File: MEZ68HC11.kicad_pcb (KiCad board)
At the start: 2 copper layers, 99.1 x 85.2 mm, 29 parts, among them J1 Conn_01x20_Socket, J2 Conn_01x20_Socket, J3 Barrel_Jack_Switch, J4 Conn_01x06_Pin, J5 Conn_01x08_Pin, J7 PinHeader_1x06_P2.54mm_Vertic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, SW1 SW_SPDT, SW2 SW_SPST, U1 PIC18F47Q43-IP, U2 628128

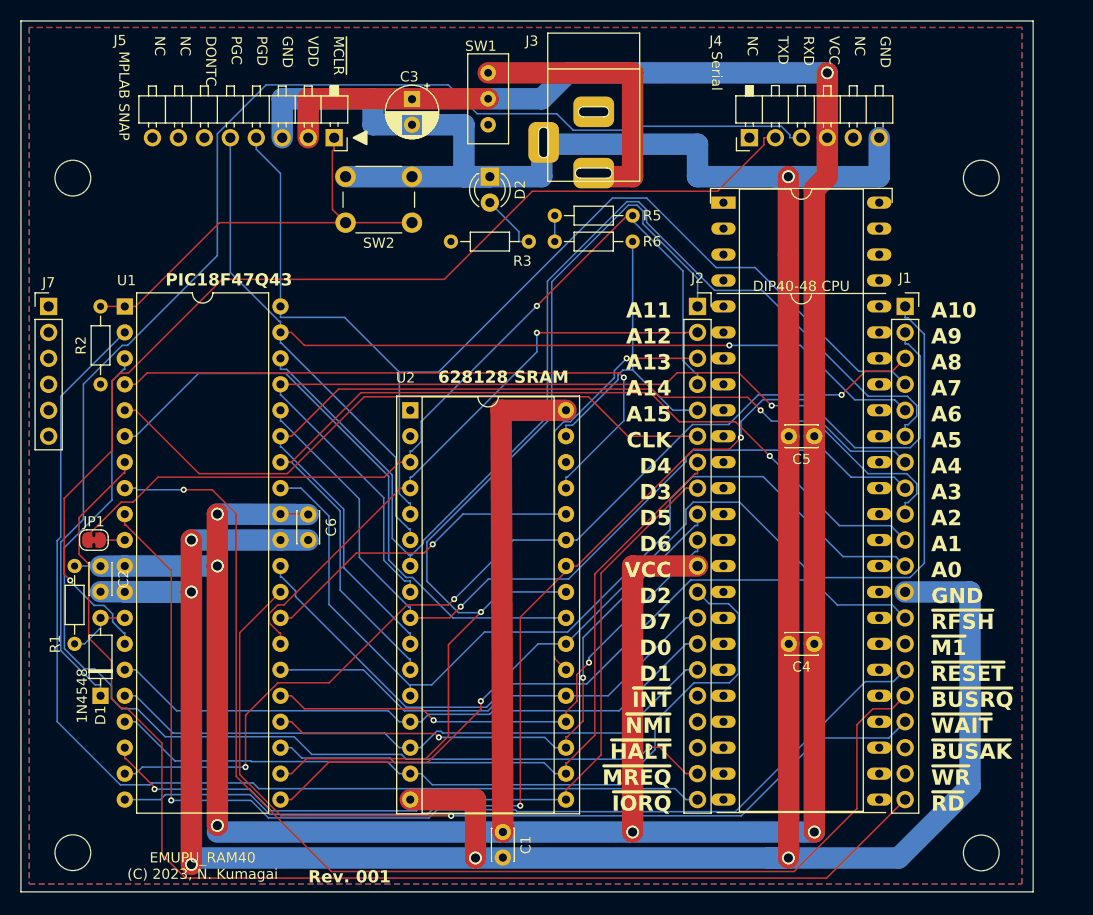
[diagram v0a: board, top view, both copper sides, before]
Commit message: Rev001. ordered to JCLPCB
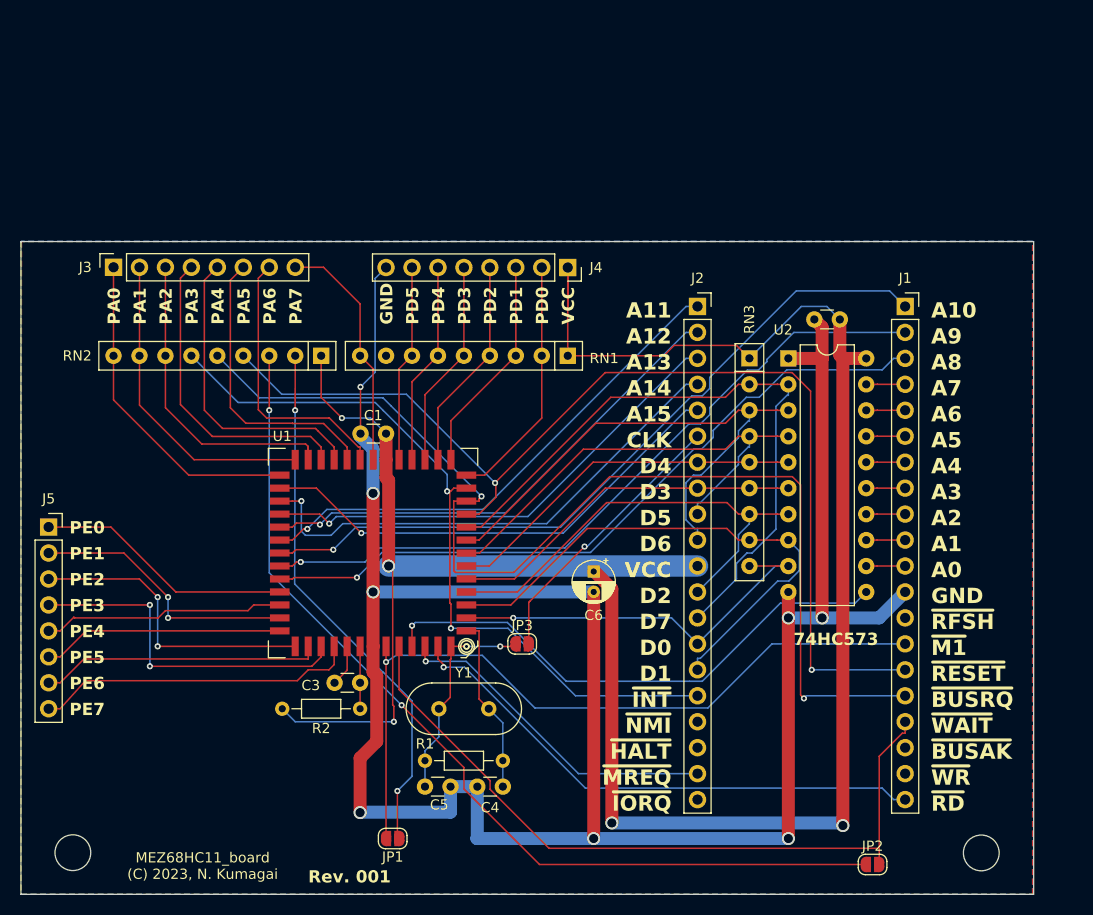
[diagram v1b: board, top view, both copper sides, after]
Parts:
- removed D1: 1N4148, Diode_THT:D_DO-35_SOD27_P7.62mm_Horizontal
- removed D2: LED, LED_THT:LED_D3.0mm
- removed DIP40-48 CPU: DIP-48_W15.24mm_Socket_OvalPad_nocourtyard, 0-local:DIP-48_W15.24mm_Socket_OvalPad_splitcouryard
- removed H5, H6: MountingHole, MountingHole:MountingHole_3.5mm
- removed J7: PinHeader_1x06_P2.54mm_Vertical, Connector_PinHeader_2.54mm:PinHeader_1x06_P2.54mm_Vertical
- removed R3: 1.5k, Resistor_THT:R_Axial_DIN0204_L3.6mm_D1.6mm_P7.62mm_Horizontal
- removed R5, R6: 10k, Resistor_THT:R_Axial_DIN0204_L3.6mm_D1.6mm_P7.62mm_Horizontal
- removed SW1: SW_SPDT, 0-local:PowerSW_for_SBC_series
- removed SW2: SW_SPST, 0-local:SW_PUSH_6mm_H4.3mm
- added JP2: SolderJumper_2_Open, Jumper:SolderJumper-2_P1.3mm_Open_RoundedPad1.0x1.5mm, F.Cu at (173.3, 148.6)
- added JP3: SolderJumper_2_Open, Jumper:SolderJumper-2_P1.3mm_Open_RoundedPad1.0x1.5mm, F.Cu at (139.1, 127.0)
- added RN1: 10kx8, Resistor_THT:R_Array_SIP9, F.Cu at (143.5, 98.8)
- added RN2: 10kx8, Resistor_THT:R_Array_SIP9, F.Cu at (119.4, 98.8)
- added RN3: 10kx8, Resistor_THT:R_Array_SIP9, F.Cu at (161.3, 99.1)
- added Y1: 8MHz, Crystal:Crystal_HC49-U_Vertical, F.Cu at (130.9, 133.3)
- C1, C2: footprint Capacitor_THT:C_Disc_D3.0mm_W2.0mm_P2.50mm -> Capacitor_THT:C_Disc_D3.0mm_W1.6mm_P2.50mm
- C3: value 10uF -> 0.1uF; footprint Capacitor_THT:CP_Radial_D5.0mm_P2.50mm -> Capacitor_THT:C_Disc_D3.0mm_W1.6mm_P2.50mm
- C4, C5: value 0.1uF -> 22pF; footprint Capacitor_THT:C_Disc_D3.0mm_W2.0mm_P2.50mm -> Capacitor_THT:C_Disc_D3.0mm_W1.6mm_P2.50mm
- C6: value 0.1uF -> 10uF; footprint Capacitor_THT:C_Disc_D3.0mm_W2.0mm_P2.50mm -> Capacitor_THT:CP_Radial_D4.0mm_P2.00mm
- J3: value Barrel_Jack_Switch -> Conn_01x08_Socket; footprint 0-local:BARREL_JACK -> Connector_PinSocket_2.54mm:PinSocket_1x08_P2.54mm_Vertical
- J4: value Conn_01x06_Pin -> Conn_01x08_Socket; footprint 0-local:PinHeader_1x06_P2.54mm_Horizontal_NoFeet -> Connector_PinSocket_2.54mm:PinSocket_1x08_P2.54mm_Vertical
- J5: value Conn_01x08_Pin -> Conn_01x08_Socket; footprint 0-local:PinHeader_1x08_P2.54mm_Rev_Horizontal_Nofoot -> Connector_PinSocket_2.54mm:PinSocket_1x08_P2.54mm_Vertical
- JP1: value SolderJumper_2_Bridged -> SolderJumper_2_Open; footprint Jumper:SolderJumper-2_P1.3mm_Bridged_RoundedPad1.0x1.5mm -> Jumper:SolderJumper-2_P1.3mm_Open_RoundedPad1.0x1.5mm
- R1: value 10k -> 10M
- R2: value 10k -> 1k
- U1: value PIC18F47Q43-IP -> 68HC11_PLCC; footprint Package_DIP:DIP-40_W15.24mm -> Package_LCC:PLCC-52
- U2: value 628128 -> 74HC573; footprint Package_DIP:DIP-32_W15.24mm_Socket -> Package_DIP:DIP-20_W7.62mm
- moved C2 76.3 mm to (170.1, 95.2), turned to 180 degrees
- moved C3 57.6 mm to (120.7, 130.8), turned to 0 degrees
- moved C5 51.3 mm to (129.5, 141.0), turned to 0 degrees
- moved J3 49.4 mm to (99.1, 90.1), turned to 90 degrees
- moved R1 46.0 mm to (137.2, 138.4), turned to 180 degrees
- moved JP1 41.3 mm to (126.4, 146.1), turned to 180 degrees
- moved R2 40.7 mm to (123.2, 133.3), turned to 180 degrees
- moved C1 40.6 mm to (125.7, 106.4), turned to 180 degrees
- moved J5 39.4 mm to (92.7, 115.6), turned to 0 degrees
- moved U2 37.3 mm to (165.1, 99.1)
- moved U1 34.2 mm to (124.5, 118.1), turned to 180 degrees
- moved C4 33.5 mm to (137.2, 141.0)
- moved C6 28.5 mm to (146.1, 119.9)
- moved J4 21.8 mm to (143.5, 90.2), turned to -90 degrees
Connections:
- C3 pad 1: VCC -> Net-(U1-VRL)
- C3 pad 2: GND -> Net-(U1-VRH)
- C4 pad 1: VCC -> Net-(U1-XTAL)
- C5 pad 1: VCC -> Net-(JP3-A)
- J3 pad 1: Net-(SW1-C) -> /PA0
- J3 pad 2: GND -> /PA1
- J3 pad 3: unconnected-(J3-Pad3) -> /PA2
- J4 pad 1: unconnected-(J4-Pin_1-Pad1) -> VCC
- J4 pad 3: Net-(D1-K) -> Net-(J4-Pin_3)
- J4 pad 4: VCC -> Net-(J4-Pin_4)
- J4 pad 5: unconnected-(J4-Pin_5-Pad5) -> Net-(J4-Pin_5)
- J4 pad 6: GND -> Net-(J4-Pin_6)
- J5 pad 2: VCC -> Net-(J5-Pin_2)
- J5 pad 3: GND -> Net-(J5-Pin_3)
- J5 pad 4: /A7 -> Net-(J5-Pin_4)
- J5 pad 5: /A6 -> Net-(J5-Pin_5)
- J5 pad 6: unconnected-(J5-Pin_6-Pad6) -> Net-(J5-Pin_6)
- J5 pad 7: unconnected-(J5-Pin_7-Pad7) -> Net-(J5-Pin_7)
- J5 pad 8: unconnected-(J5-Pin_8-Pad8) -> Net-(J5-Pin_8)
- JP1 pad 1: /A14 -> Net-(JP1-A)
- JP1 pad 2: Net-(JP1-B) -> /~{M1}
- R1 pad 1: VCC -> Net-(U1-XTAL)
- R1 pad 2: Net-(D1-A) -> Net-(JP3-A)
- R2 pad 1: VCC -> Net-(U1-VRH)
- R2 pad 2: Net-(J5-Pin_1) -> VCC
- U1 pad 1: Net-(J5-Pin_1) -> GND
- U1 pad 10: Net-(JP1-B) -> /D1
- U1 pad 11: VCC -> /D2
- U1 pad 12: GND -> /D3
- U1 pad 13: Net-(D1-A) -> /D4
- U1 pad 14: Net-(J4-Pin_2) -> /D5
- U1 pad 15: /D0 -> /D6
- U1 pad 16: /D1 -> /D7
- U1 pad 17: /D2 -> /~{RESET}
- U1 pad 18: /D3 -> /~{BUSRQ}
- U1 pad 19: /A8 -> /~{INT}
- U1 pad 2: /~{IORQ} -> /~{M1}
- U1 pad 20: /A9 -> Net-(J4-Pin_2)
- U1 pad 21: /A10 -> Net-(J4-Pin_3)
- U1 pad 22: /A11 -> Net-(J4-Pin_4)
- U1 pad 23: /D4 -> Net-(J4-Pin_5)
- U1 pad 24: /D5 -> Net-(J4-Pin_6)
- U1 pad 25: /D6 -> Net-(J4-Pin_7)
- U1 pad 26: /D7 -> VCC
- U1 pad 27: /A12 -> /PA7
- U1 pad 28: /A13 -> Net-(J3-Pin_7)
- U1 pad 29: /~{WAIT} -> Net-(J3-Pin_6)
- U1 pad 3: /~{MREQ} -> /~{WAIT}
- U1 pad 30: /~{RFSH} -> Net-(J3-Pin_5)
- U1 pad 31: GND -> Net-(J3-Pin_4)
- U1 pad 32: VCC -> /PA2
- U1 pad 33: /A0 -> /PA1
- U1 pad 34: /A1 -> /PA0
- U1 pad 35: /A2 -> /A15
- U1 pad 36: /A3 -> /A14
- U1 pad 37: /A4 -> /A13
- U1 pad 38: /A5 -> /A12
- U1 pad 39: /A6 -> /A11
- U1 pad 4: Net-(U1-RA2) -> Net-(U1-AS)
- U1 pad 40: /A7 -> /A10
- U1 pad 5: /CLK -> /~{MREQ}
- U1 pad 6: Net-(U1-RA4) -> /~{RD}
- U1 pad 7: /~{RD} -> Net-(JP3-A)
- U1 pad 8: /~{BUSRQ} -> Net-(U1-XTAL)
- U1 pad 9: /~{RESET} -> /D0
- U2 pad 1: unconnected-(U2-NC-Pad1) -> GND
- U2 pad 10: /A2 -> GND
- U2 pad 11: /A1 -> Net-(U1-AS)
- U2 pad 13: /D0 -> /A1
- U2 pad 14: /D1 -> /A2
- U2 pad 15: /D2 -> /A3
- U2 pad 16: GND -> /A4
- U2 pad 17: /D3 -> /A5
- U2 pad 18: /D4 -> /A6
- U2 pad 19: /D5 -> /A7
- U2 pad 2: VCC -> /D7
- U2 pad 20: /D6 -> VCC
- U2 pad 3: /A14 -> /D6
- U2 pad 4: /A12 -> /D5
- U2 pad 5: /A7 -> /D4
- U2 pad 6: /A6 -> /D3
- U2 pad 7: /A5 -> /D2
- U2 pad 8: /A4 -> /D1
- U2 pad 9: /A3 -> /D0
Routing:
- net Net-(D1-K): track 125.3 -> 0.00 mm
- net GND: track 341.8 -> 220.5 mm, vias 6 -> 8
- net /A6: track 111.2 -> 3.81 mm, vias 1 -> 0
- net /A7: track 110.9 -> 3.81 mm
- net /~{IORQ}: track 106.8 -> 0.00 mm
- net /A5: track 110.4 -> 3.81 mm
- net VCC: track 326.7 -> 224.8 mm, vias 6 -> 5
- net /A2: track 97.4 -> 3.81 mm, vias 1 -> 0
- net Net-(JP2-A): track 0.00 -> 92.7 mm, vias 0 -> 2
- net /A1: track 96.2 -> 3.81 mm, vias 1 -> 0
- net /A4: track 91.2 -> 3.81 mm, vias 1 -> 0
- net /A0: track 89.0 -> 3.81 mm
- net Net-(J4-Pin_2): track 105.9 -> 24.4 mm, vias 1 -> 0
- net /A3: track 82.7 -> 3.81 mm, vias 1 -> 0
- net /~{M1}: track 0.00 -> 74.5 mm, vias 0 -> 1
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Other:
- board size 99.1 x 85.2 mm -> 99.1 x 63.9 mm
- board text added: "74HC573"
- board text added: "MEZ68HC11_board (C) 2023, N. Kumagai"
- board text added: "PA0"
- board text added: "PA1"
- board text added: "PA2"
- board text added: "PA3"
- board text added: "PA4"
- board text added: "PA5"
- board text added: "PA6"
- board text added: "PA7"
- board text added: "PD0"
- board text added: "PD1"
- board text added: "PD2"
- board text added: "PD3"
- board text added: "PD4"
- board text added: "PD5"
- board text added: "PE0"
- board text added: "PE1"
- board text added: "PE2"
- board text added: "PE3"
- board text added: "PE4"
- board text added: "PE5"
- board text added: "PE6"
- board text added: "PE7"
- board text removed: "628128 SRAM"
- board text removed: "DONTC"
- board text removed: "EMUPU_RAM40 (C) 2023, N. Kumagai"
- board text removed: "MPLAB SNAP"
- board text removed: "NC"
- board text removed: "PGC"
- board text removed: "PGD"
- board text removed: "PIC18F47Q43"
- board text removed: "RXD"
- board text removed: "Serial"
- board text removed: "TXD"
- board text removed: "VDD"
- board text removed: "~{MCLR}"
